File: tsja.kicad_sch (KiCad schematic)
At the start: 68 parts, among them J1 QWIIC, J2 Micro_SD_Card, J3 SAO, J4 EXT, J6 USB-C, M1 Vibration, Q1 AP2302B, Q4 AO3400 (A09T), Q5 AO3400 (A09T), T1 Select, T2 Start, T3 B, T4 A, T5 Cross, U1 74LVC1G17GW,125, U10 SY6280AAC, U11 SK6805, U12 SK6805, U13 SK6805, U14 SK6805, U15 SK6805, U2 MPR121QR2, U3 ESP32-WROVER-E, U7 CH340K, U8 SK6805, U9 SY6280AAC

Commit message: Cleanup & tweaks
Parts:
- C2, C24, C3: LCSC C307331 -> (none)
- C26, C27: Buy early Y -> (none); Category Capacitors -> (none); LCSC C602037 -> (none); MPN CL21A226MAYNNNE -> (none); Manufacturer Samsung Electro-Mechanics -> (none); Minimal voltage rating 10 -> (none); Sponsored N -> (none); Voltage rating 25 -> (none)
- M1: footprint Connector_PinHeader_2.00mm:PinHeader_1x02_P2.00mm_Vertical -> Connector_PinHeader_2.54mm:PinHeader_1x02_P2.54mm_Vertical_SMD_Pin1Left
- R6, R7: LCSC C60490 -> (none)
- U10: Buy early Y -> (none); Category ICs -> (none); MPN SY6280AAC -> (none); Manufacturer Silergy Corp -> (none); Mouser - -> (none); Sponsored N -> (none)

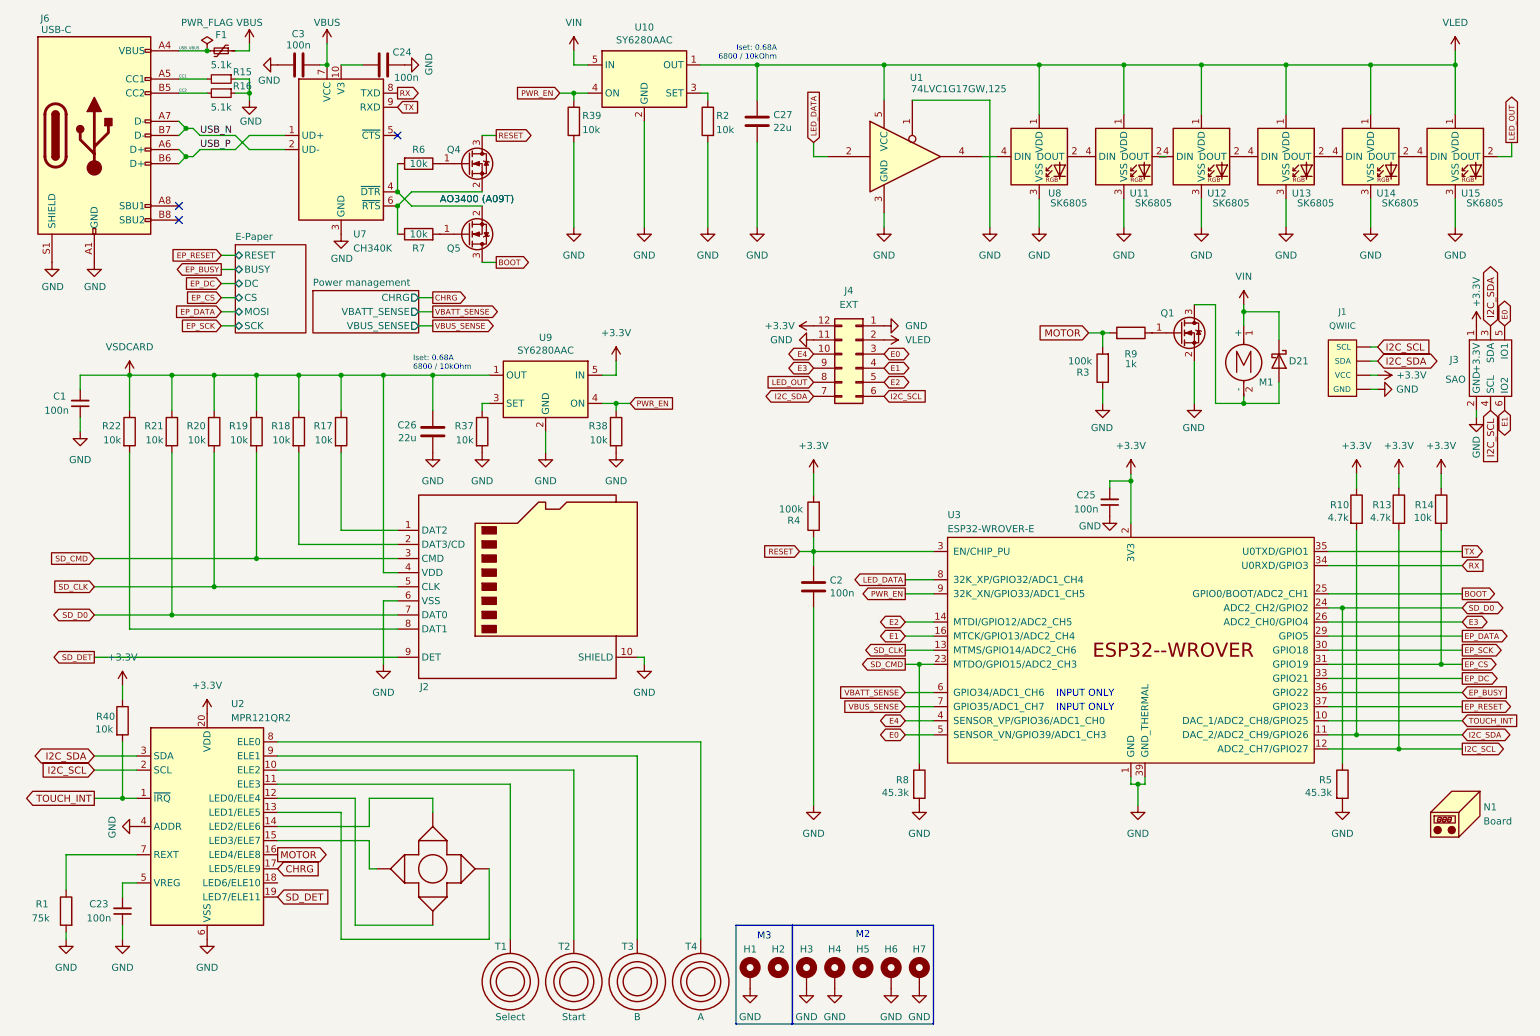
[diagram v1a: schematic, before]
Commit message: Apply fixes proposed by Paul
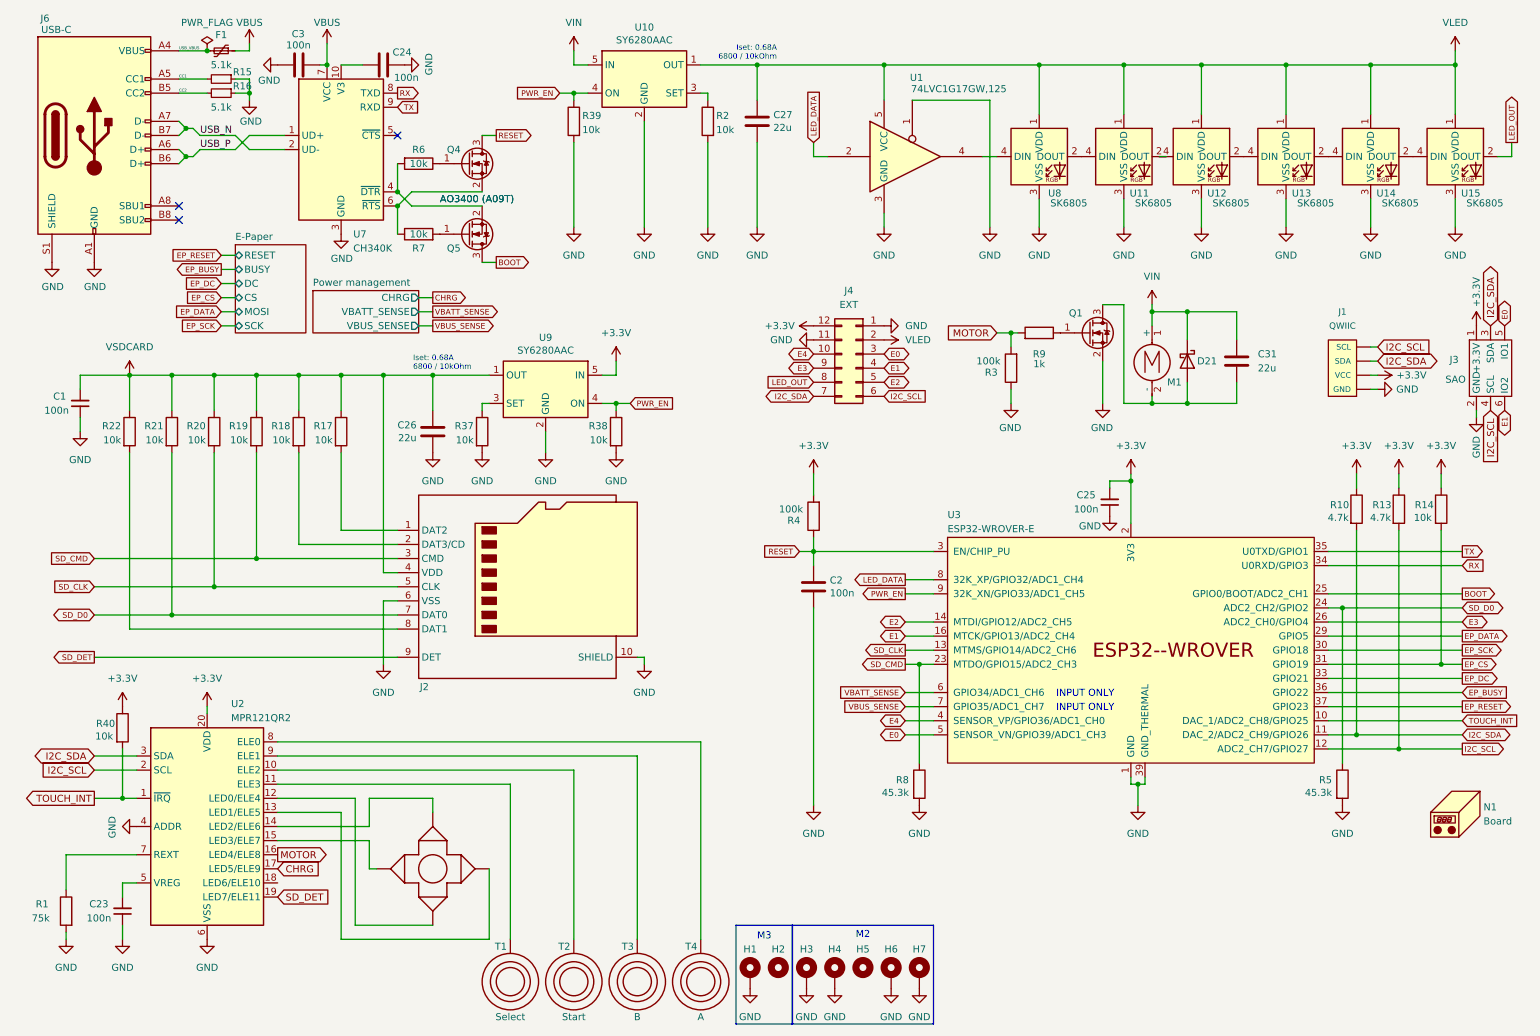
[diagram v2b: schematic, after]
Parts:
- added C31: 22u, Capacitor_SMD:C_0805_2012Metric, symbol Device:C
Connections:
- net VIN: now also C31.1
- net at D21.2 (A), M1.2 (-), Q1.3 (D): now also C31.2
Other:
- moved on the sheet: D21, M1, Q1, R3, R40, R9
